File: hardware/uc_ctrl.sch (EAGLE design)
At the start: 31 parts, among them Q4 si2305cd, Q7 si2305cd, T1 BC846, T3 BC846, Y1 32768Hz CFPX-217 12.5pF

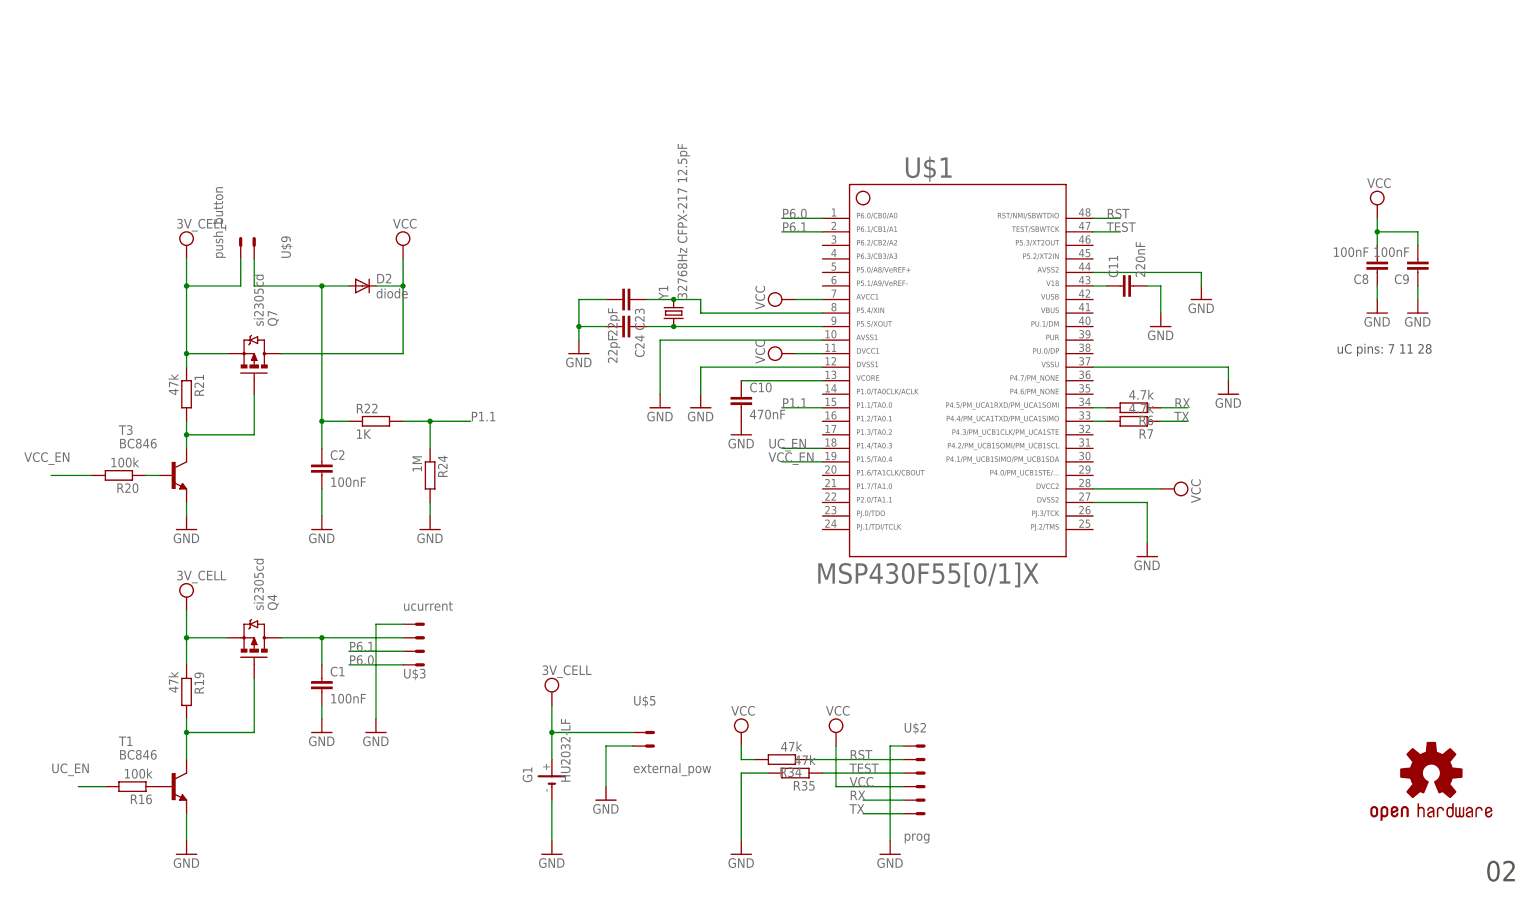
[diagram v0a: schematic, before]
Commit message: rev 2
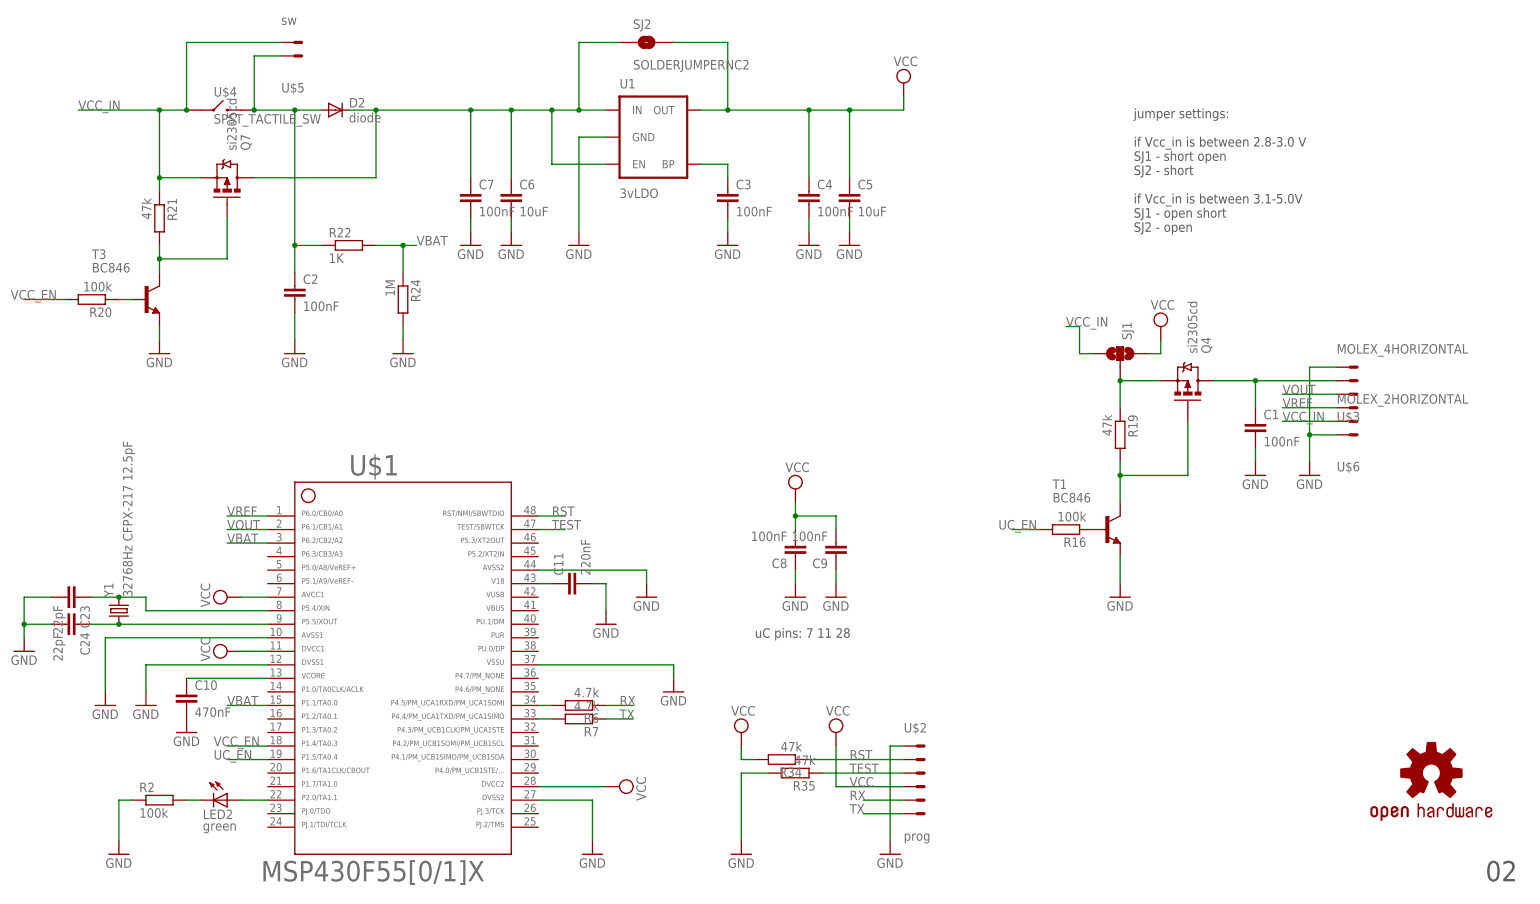
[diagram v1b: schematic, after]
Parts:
- removed G1: HU2032-LF, Simplex-Battery:HU2032-LF
- removed U$9: push_button, Simplex-Connectors:MOLEX_2VERTICAL
- added C3, C4, C7: 100nF, rcl:C-EUC0805
- added C5, C6: 10uF, rcl:C-EUC0805
- added LED2: green, led:LEDCHIPLED_0805
- added R2: 100k, rcl:R-EU_R0805W
- added SJ1: (no value), SparkFun-Passives:SOLDERJUMPER_2WAYPASTE1&2
- added SJ2: SOLDERJUMPERNC2, SparkFun-Passives:SOLDERJUMPERNC2
- added U$4: SPST_TACTILE_SW, Simplex-Switches:SPST_TACTILE_SW
- added U$6: MOLEX_2HORIZONTAL, Simplex-Connectors:MOLEX_2HORIZONTAL
- added U1: 3vLDO, SparkFun-PowerIC:V_REG_LDOSMD
- U$2: device Simplex-Connectors:MOLEX_6VERTICAL -> Simplex-Connectors:MOLEX_6HORIZONTAL
- U$3: value ucurrent -> MOLEX_4HORIZONTAL; device Simplex-Connectors:MOLEX_4VERTICAL -> Simplex-Connectors:MOLEX_4HORIZONTAL
- U$5: value external_pow -> sw; device Simplex-Connectors:MOLEX_2VERTICAL -> Simplex-Connectors:MOLEX_2HORIZONTAL
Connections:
- net P6.0 renamed VREF
- net P6.1 renamed VOUT
- removed net 3V_CELL: G1.+, Q4.S, Q7.S, R19.1, R21.1, U$5.1, U$9.2
- removed net P1.1: R22.2, R24.1, U$1.15
- new net N$1: LED2.C, R2.2
- new net N$2: LED2.A, U$1.22
- new net N$4: C6.1, C7.1, D2.C, Q7.D, SJ2.1, U1.EN, U1.IN
- new net N$5: C3.1, U1.BP
- new net N$8: Q4.S, R19.1, SJ1.2
- new net VBAT: R22.2, R24.1, U$1.15, U$1.3
- new net VCC_IN: Q7.S, R21.1, SJ1.3, U$4.1, U$5.2, U$6.2
- net GND: now also C3.2, C4.2, C5.2, C6.2, C7.2, R2.1, U$6.1, U1.GND; no longer G1.-, U$5.2
- net PUSH: now also U$4.2, U$5.1; no longer U$9.1
- net UC_EN: now also U$1.19; no longer U$1.18
- net VCC: now also C4.1, C5.1, SJ1.1, SJ2.2, U1.OUT; no longer D2.C, Q7.D
- net VCC_EN: now also U$1.18; no longer U$1.19
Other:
- note added: "jumper settings: if Vcc_in is between 2.8-3.0 V SJ1 - short open SJ2 - short if Vcc_in is between 3.1-5.0V SJ1 - open short SJ2 - open"
- moved on the sheet: C1, C10, C11, C2, C23, C24, C8, C9, D2, Q4, Q7, R16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
